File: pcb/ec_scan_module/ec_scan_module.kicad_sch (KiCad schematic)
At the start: 17 parts, among them J2 Conn_01x08, J3 Conn_01x08, U2 TLV9061IDBVR, U3 74HC4051

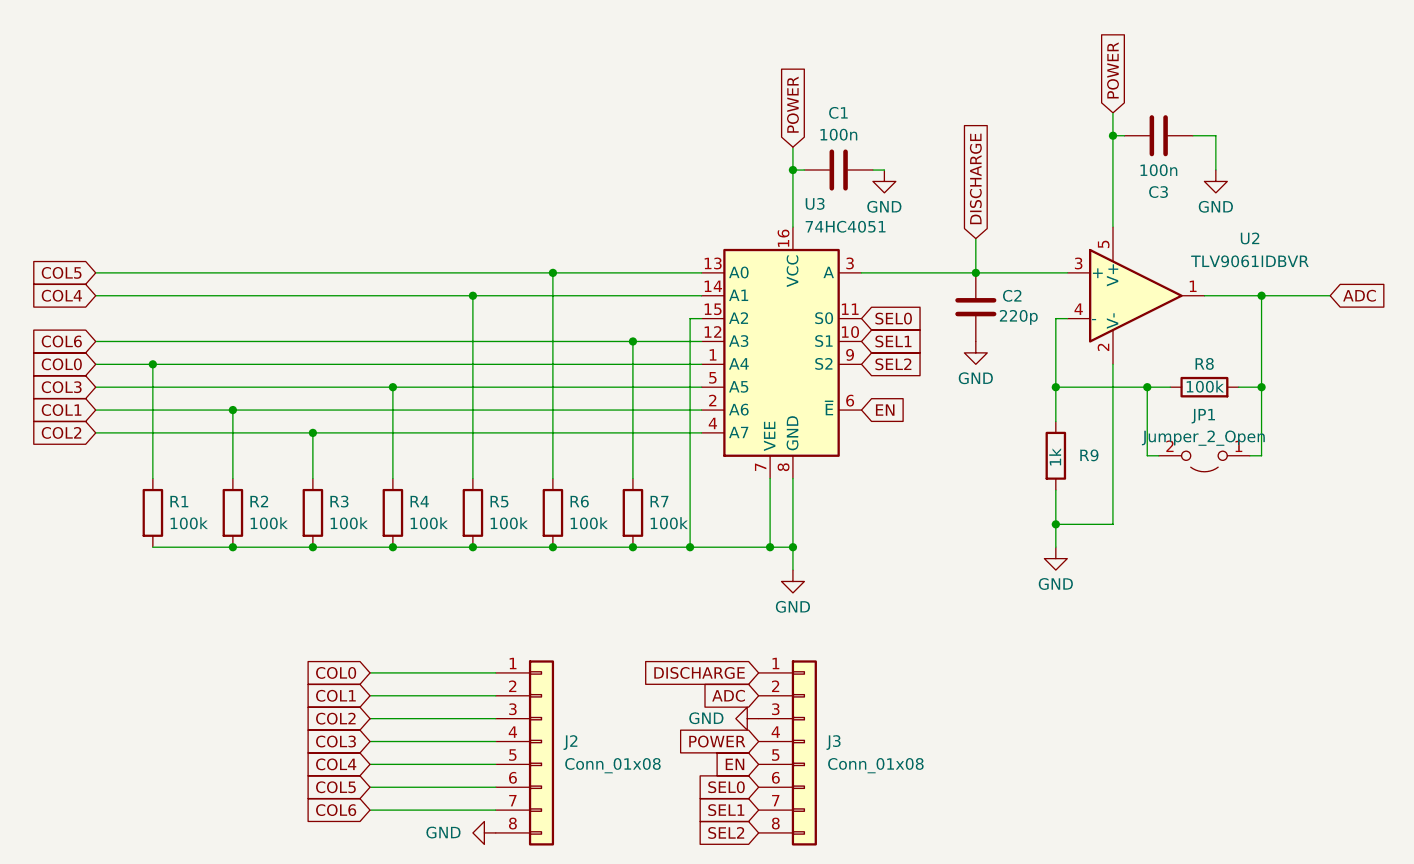
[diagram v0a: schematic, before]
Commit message: modify
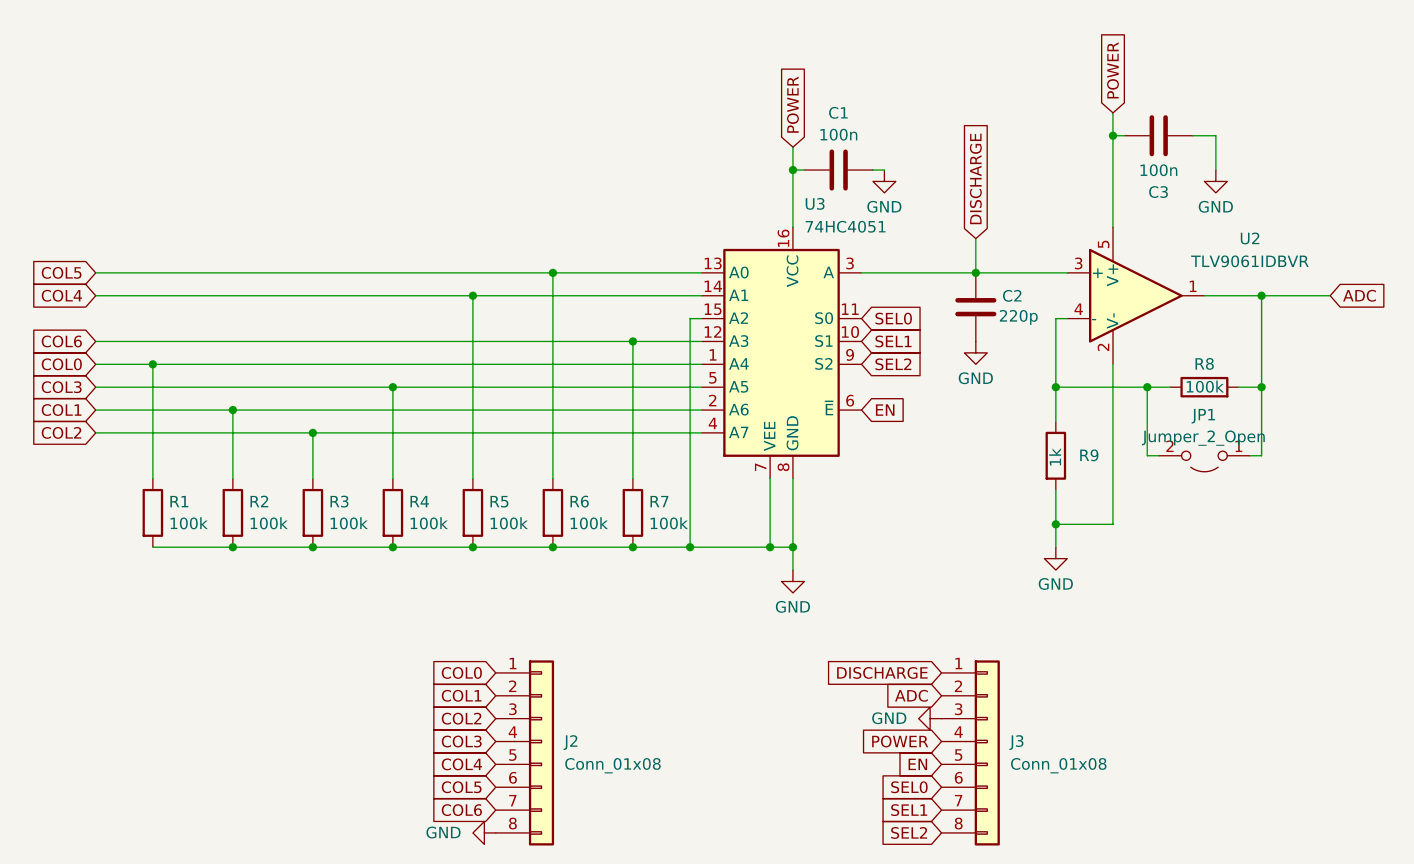
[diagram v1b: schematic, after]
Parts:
- C1, C2, C3: footprint Capacitor_SMD:C_0805_2012Metric_Pad1.18x1.45mm_HandSolder -> Capacitor_SMD:C_0402_1005Metric
- JP1: footprint Resistor_SMD:R_0805_2012Metric_Pad1.20x1.40mm_HandSolder -> Resistor_SMD:R_0201_0603Metric_Pad0.64x0.40mm_HandSolder
- R1, R2, R3, R4, R5, R6, R7, R8, R9: footprint Resistor_SMD:R_0805_2012Metric_Pad1.20x1.40mm_HandSolder -> Resistor_SMD:R_0402_1005Metric
- U3: footprint Package_SO:SOIC-16_3.9x9.9mm_P1.27mm -> Package_SO:TSSOP-16_4.4x5mm_P0.65mm
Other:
- moved on the sheet: J3
